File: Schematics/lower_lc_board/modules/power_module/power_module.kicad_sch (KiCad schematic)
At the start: 29 parts, among them J1 Stack Male Edge Connector, U1 TVS3300DRV, U2 LD1117S33TR_SOT223, U3 ID_LM66100DCKR, U4 ID_LM66100DCKR

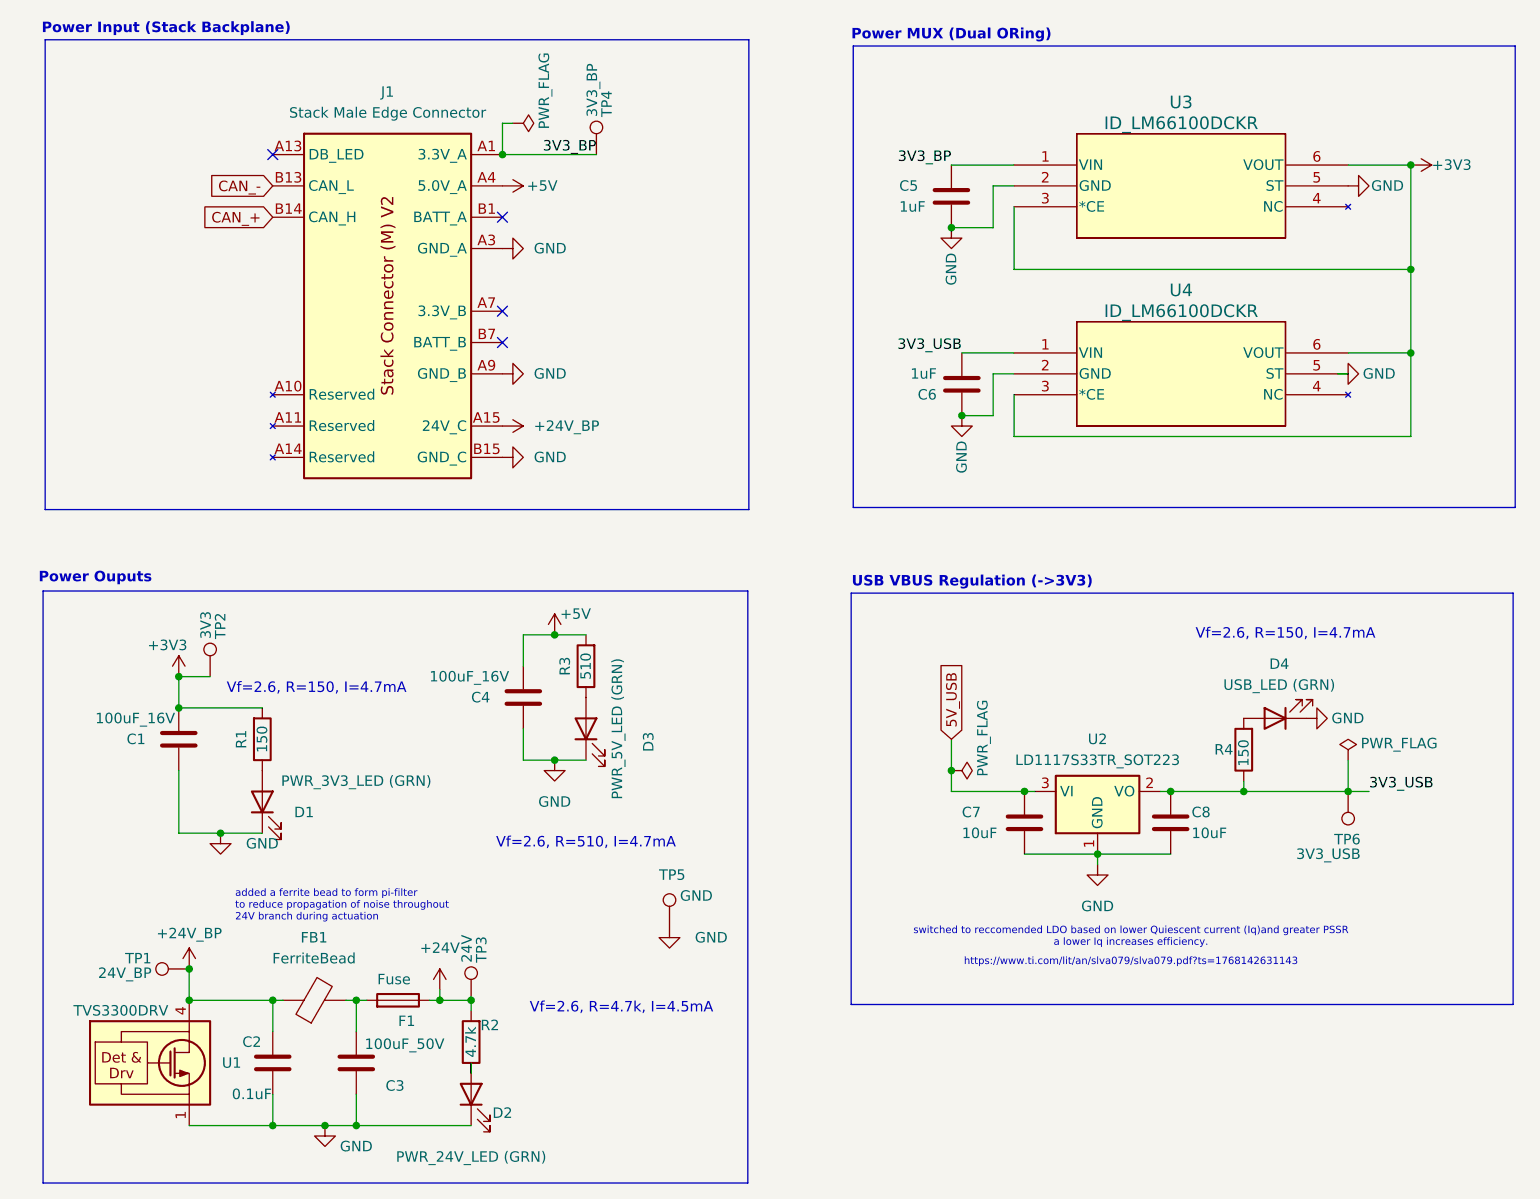
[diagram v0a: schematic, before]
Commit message: pin assignments verified
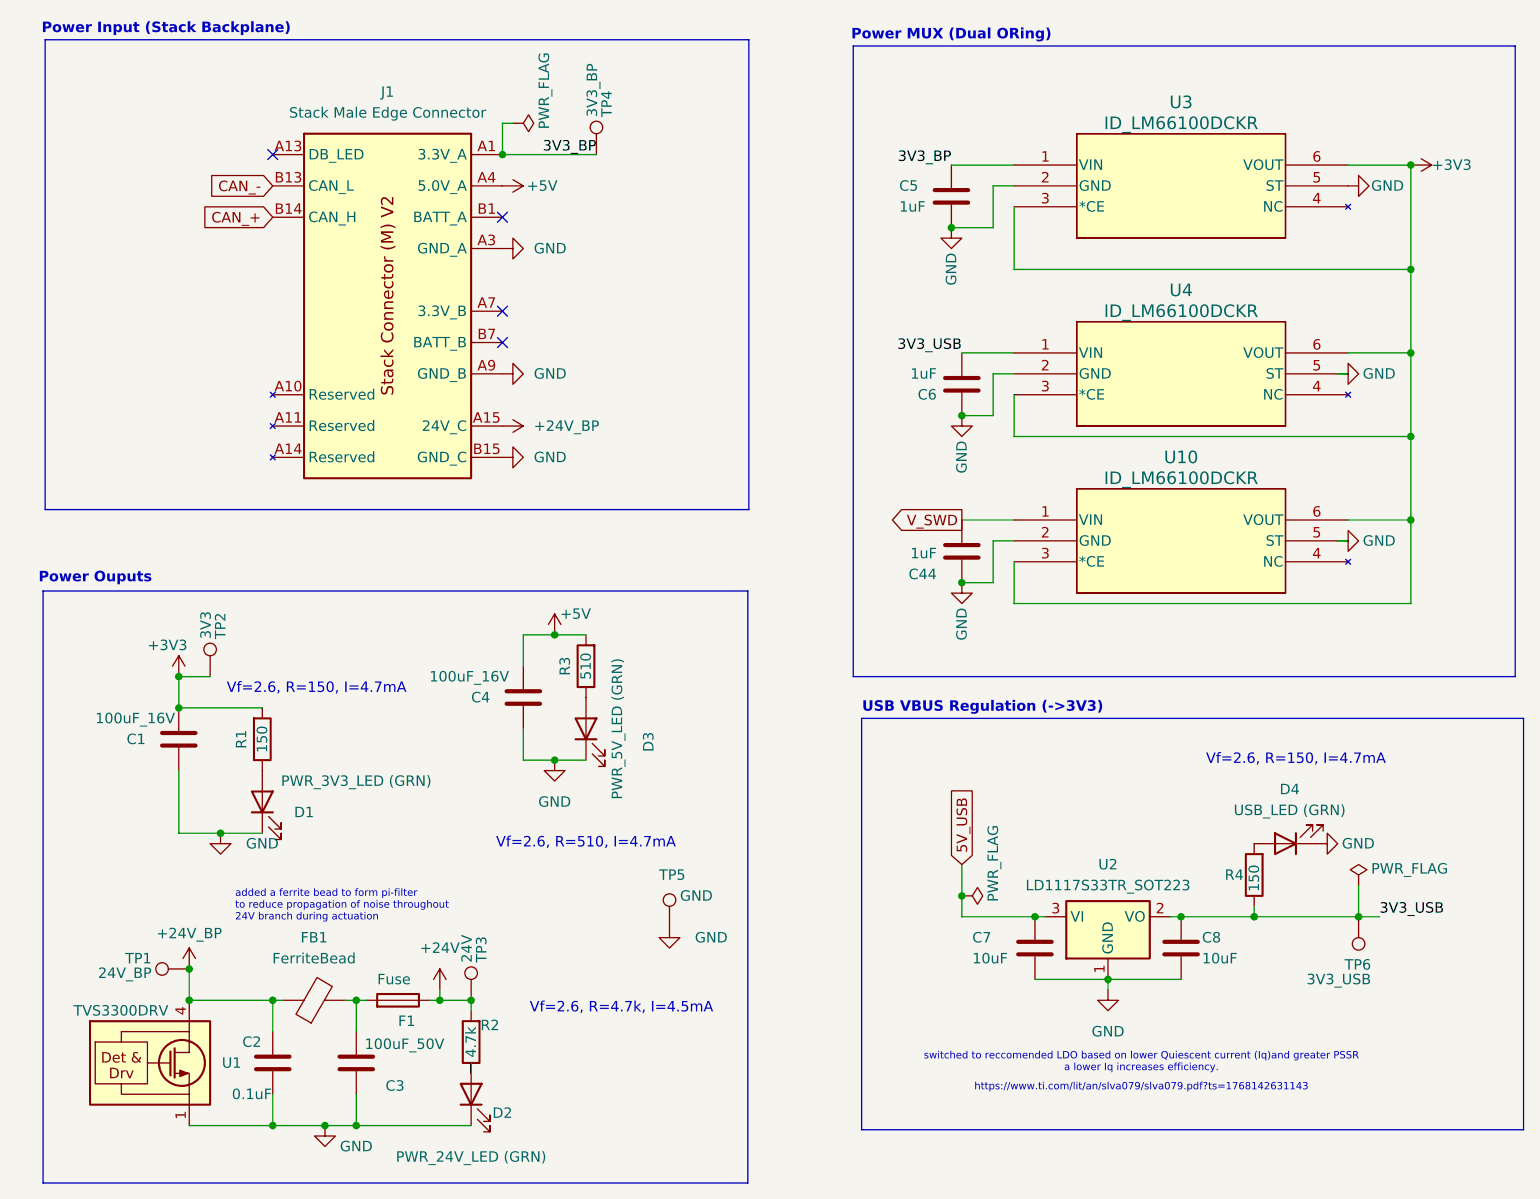
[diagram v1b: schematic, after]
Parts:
- added C44: 1uF, Capacitor_SMD:C_0603_1608Metric, symbol Device:C
- added U10: ID_LM66100DCKR, LM66100:SC-70-6, symbol QRET_Buck_PSU:LM66100DCKR
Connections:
- net +3V3: now also U10.3 (*CE), U10.6 (VOUT)
- net GND: now also C44.2, U10.2 (GND), U10.5 (ST)
- new net V_SWD: C44.1, U10.1 (VIN)
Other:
- moved on the sheet: C7, C8, D4, R4, TP6, U2
